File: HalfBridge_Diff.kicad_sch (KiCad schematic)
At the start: 8 parts, among them J5 Conn_01x04_Shielded, J7 Conn_01x02, U3 MAX3284E, U5 MAX3284E

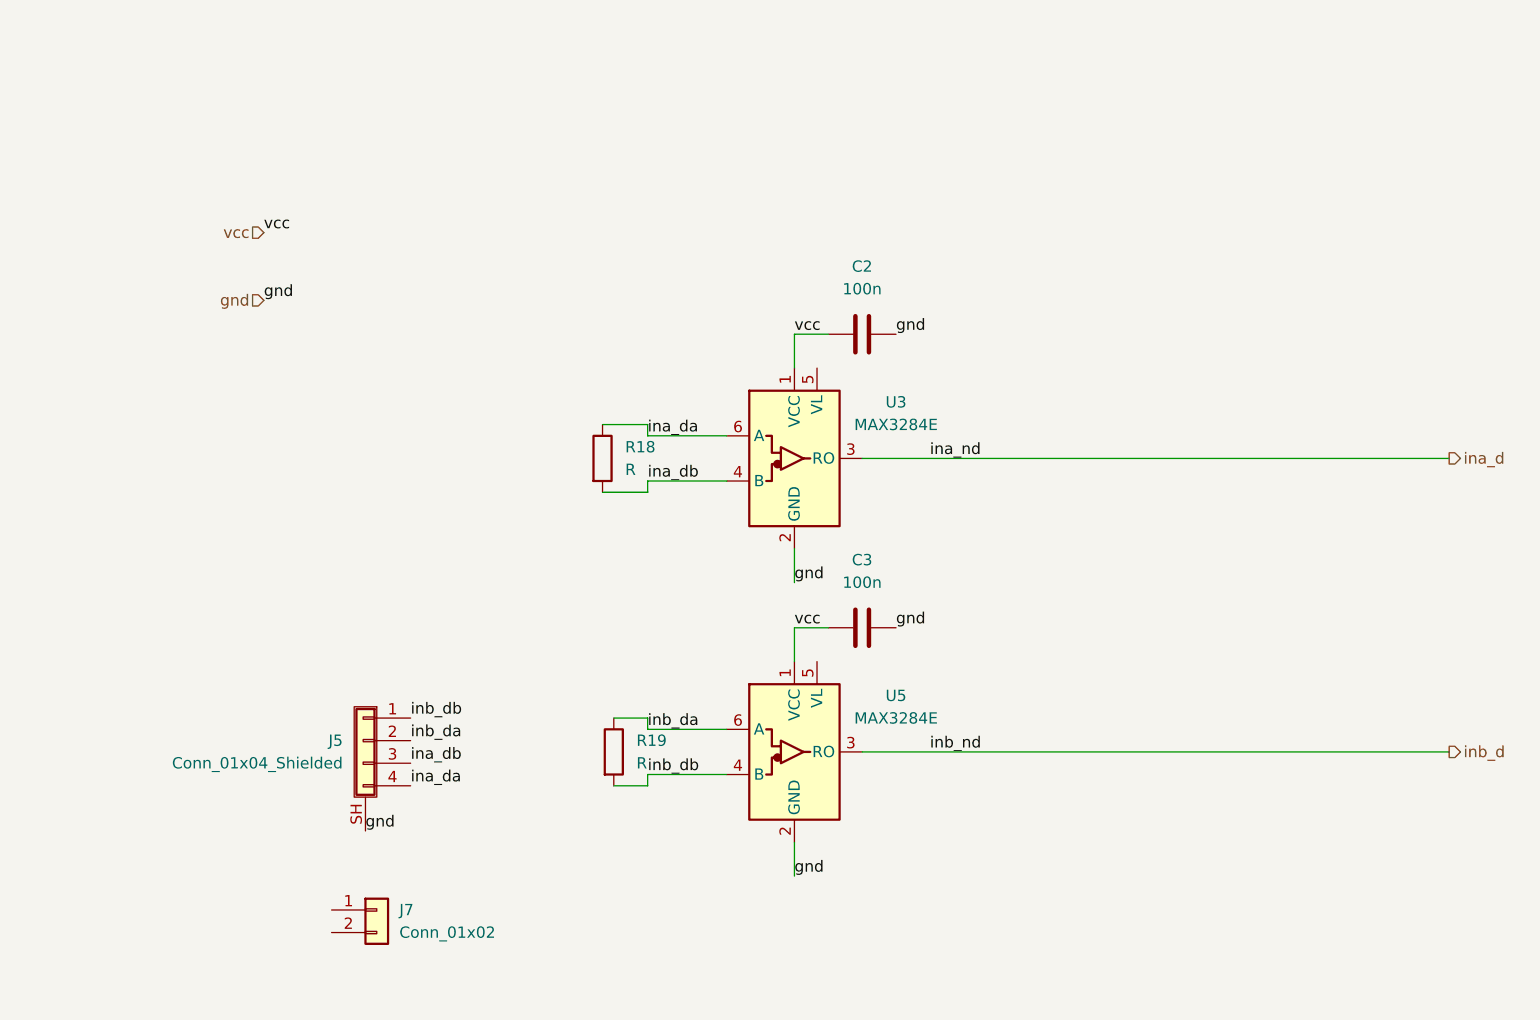
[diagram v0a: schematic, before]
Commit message: diff circuit
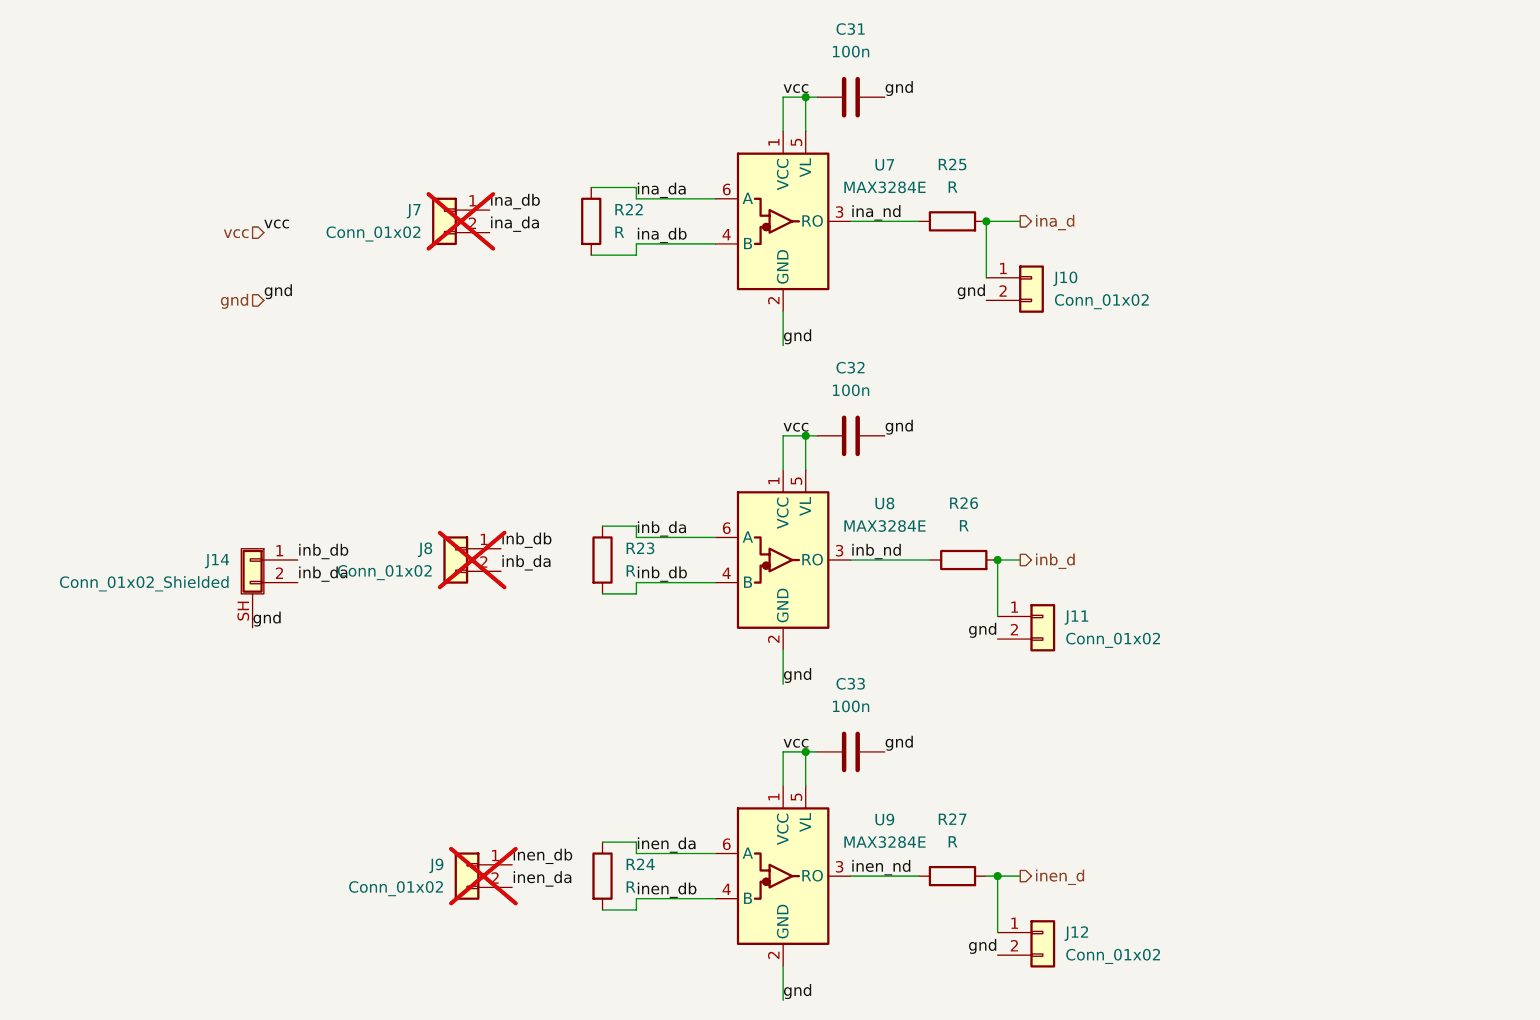
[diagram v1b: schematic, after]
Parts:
- removed J5: Conn_01x04_Shielded, My_Connector:Samtec_T1M-04-X-SH-L_1x04-1SH_P1.0mm_Terminal_Horizontal_Latch, symbol Connector_Generic_Shielded:Conn_01x04_Shielded
- added C33: 100n, Capacitor_SMD:C_0603_1608Metric_Pad1.08x0.95mm_HandSolder, symbol Device:C
- added J10, J11, J12, J8, J9: Conn_01x02, Connector_PinHeader_2.54mm:PinHeader_1x02_P2.54mm_Vertical, symbol Connector_Generic:Conn_01x02
- added J14: Conn_01x02_Shielded, My_Connector:SAMTEC_T1M-02-F-SV-L-P, symbol Connector_Generic_Shielded:Conn_01x02_Shielded
- added R24: R, Resistor_SMD:R_0603_1608Metric_Pad0.98x0.95mm_HandSolder, symbol Device:R
- added R25, R26, R27: R, Resistor_SMD:R_0603_1608Metric, symbol Device:R
- added U9: MAX3284E, Package_TO_SOT_SMD:SOT-23-6_Handsoldering, symbol Interface_UART:MAX3284E
- J7: now not fitted
- renumbered C2 to C31, C3 to C32, R18 to R22, R19 to R23, U3 to U7, U5 to U8
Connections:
- net gnd: now also C33.2, J10.2 (Pin_2), J11.2 (Pin_2), J12.2 (Pin_2), J14.SH (Shield), U9.2 (GND)
- net ina_d: now also J10.1 (Pin_1), R25.2; no longer U7.3 (RO)
- net ina_da: now also J7.2 (Pin_2)
- net ina_db: now also J7.1 (Pin_1)
- net inb_d: now also J11.1 (Pin_1), R26.2; no longer U8.3 (RO)
- net inb_da: now also J14.2 (Pin_2), J8.2 (Pin_2)
- net inb_db: now also J14.1 (Pin_1), J8.1 (Pin_1)
- net vcc: now also U7.5 (VL), U8.5 (VL), C33.1, U9.1 (VCC), U9.5 (VL)
- new net ina_nd: R25.1, U7.3 (RO)
- new net inb_nd: R26.1, U8.3 (RO)
- new net inen_d: J12.1 (Pin_1), R27.2
- new net inen_da: J9.2 (Pin_2), R24.1, U9.6 (A)
- new net inen_db: J9.1 (Pin_1), R24.2, U9.4 (B)
- new net inen_nd: R27.1, U9.3 (RO)
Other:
- moved on the sheet: C31, C32, R22, R23, U7, U8
